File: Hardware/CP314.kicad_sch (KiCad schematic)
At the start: 14 parts, among them IC1 IS63WV1288DBLL-10TLI, IC2 SN74LVC573APWRE4, IC3 SN74LVC573APWRE4, J1 Raspberry_Pi_2_3, J2 Conn_02x11_Odd_Even, U1 XC9572XL-VQ64

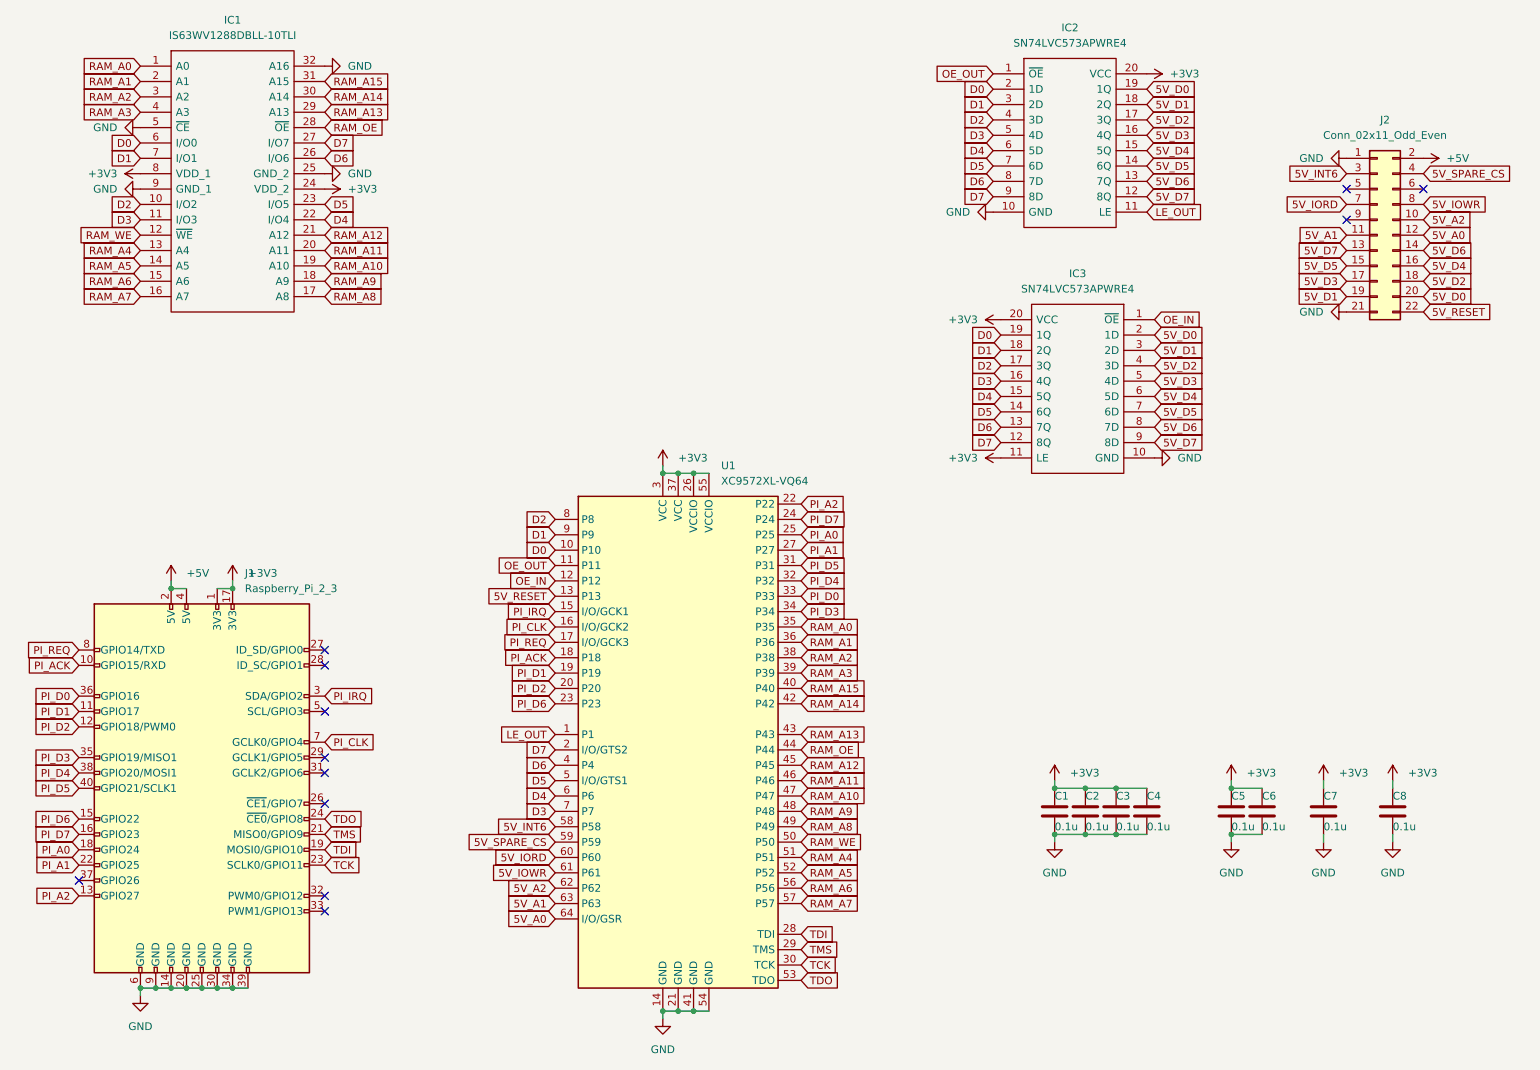
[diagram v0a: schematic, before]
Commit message: Initial file updates
PCB data replaced. Readme updated/simplified with further links to Niklas repo.
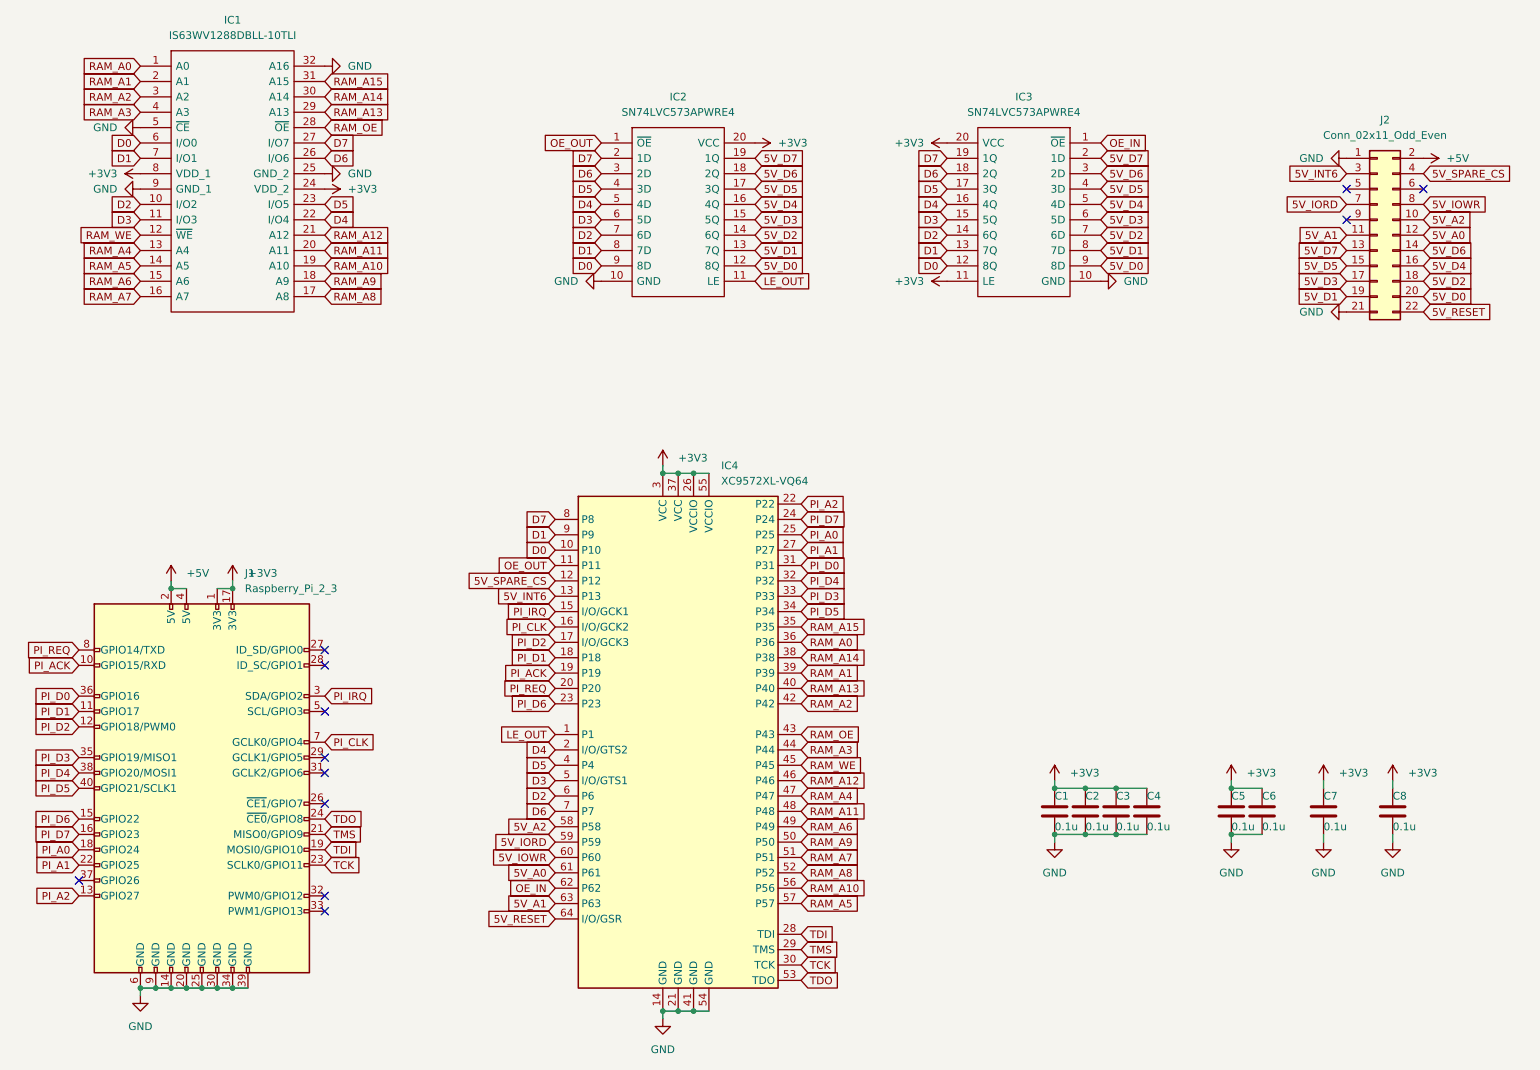
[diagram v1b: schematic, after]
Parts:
- IC1: footprint SOIC127P1176X120-32N -> Package_SO:TSOP-II-32_21.0x10.2mm_P1.27mm
- IC2, IC3: footprint SOP65P640X120-20N -> Package_SO:TSSOP-20_4.4x6.5mm_P0.65mm
- J1: footprint Connector_PinSocket_2.54mm:PinSocket_2x20_P2.54mm_Vertical -> Adafruit:ADA3708_RPI-ZERO_NO_HOLES; symbol Connector:Raspberry_Pi_2_3 -> Adafruit:Raspberry Pi; MANUFACTURER (none) -> Raspberry Pi Foundation
- J2: footprint Connector_PinSocket_2.00mm:PinSocket_2x11_P2.00mm_Vertical -> Connector_PinSocket_2.00mm:PinSocket_2x11_P2.00mm_Vertical_SMD
- renumbered U1 to IC4
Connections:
- net 5V_A0: now also IC4.61 (P61); no longer IC4.64 (I/O/GSR)
- net 5V_A2: now also IC4.58 (P58); no longer IC4.62 (P62)
- net 5V_D0: now also IC2.12 (8Q), IC3.9 (8D); no longer IC2.19 (1Q), IC3.2 (1D)
- net 5V_D1: now also IC2.13 (7Q), IC3.8 (7D); no longer IC2.18 (2Q), IC3.3 (2D)
- net 5V_D2: now also IC2.14 (6Q), IC3.7 (6D); no longer IC2.17 (3Q), IC3.4 (3D)
- net 5V_D3: now also IC2.15 (5Q), IC3.6 (5D); no longer IC2.16 (4Q), IC3.5 (4D)
- net 5V_D4: now also IC2.16 (4Q), IC3.5 (4D); no longer IC2.15 (5Q), IC3.6 (5D)
- net 5V_D5: now also IC2.17 (3Q), IC3.4 (3D); no longer IC2.14 (6Q), IC3.7 (6D)
- net 5V_D6: now also IC2.18 (2Q), IC3.3 (2D); no longer IC2.13 (7Q), IC3.8 (7D)
- net 5V_D7: now also IC2.19 (1Q), IC3.2 (1D); no longer IC2.12 (8Q), IC3.9 (8D)
- net 5V_INT6: now also IC4.13 (P13); no longer IC4.58 (P58)
- net 5V_IORD: now also IC4.59 (P59); no longer IC4.60 (P60)
- net 5V_IOWR: now also IC4.60 (P60); no longer IC4.61 (P61)
- net 5V_RESET: now also IC4.64 (I/O/GSR); no longer IC4.13 (P13)
- net 5V_SPARE_CS: now also IC4.12 (P12); no longer IC4.59 (P59)
- net D0: now also IC2.9 (8D), IC3.12 (8Q); no longer IC2.2 (1D), IC3.19 (1Q)
- net D1: now also IC2.8 (7D), IC3.13 (7Q); no longer IC2.3 (2D), IC3.18 (2Q)
- net D2: now also IC2.7 (6D), IC3.14 (6Q), IC4.6 (P6); no longer IC2.4 (3D), IC3.17 (3Q), IC4.8 (P8)
- net D3: now also IC2.6 (5D), IC3.15 (5Q), IC4.5 (I/O/GTS1); no longer IC2.5 (4D), IC3.16 (4Q), IC4.7 (P7)
- net D4: now also IC2.5 (4D), IC3.16 (4Q), IC4.2 (I/O/GTS2); no longer IC2.6 (5D), IC3.15 (5Q), IC4.6 (P6)
- net D5: now also IC2.4 (3D), IC3.17 (3Q), IC4.4 (P4); no longer IC2.7 (6D), IC3.14 (6Q), IC4.5 (I/O/GTS1)
- net D6: now also IC2.3 (2D), IC3.18 (2Q), IC4.7 (P7); no longer IC2.8 (7D), IC3.13 (7Q), IC4.4 (P4)
- net D7: now also IC2.2 (1D), IC3.19 (1Q), IC4.8 (P8); no longer IC2.9 (8D), IC3.12 (8Q), IC4.2 (I/O/GTS2)
- net OE_IN: now also IC4.62 (P62); no longer IC4.12 (P12)
- net PI_ACK: now also IC4.19 (P19); no longer IC4.18 (P18)
- net PI_D0: now also IC4.31 (P31); no longer IC4.33 (P33)
- net PI_D1: now also IC4.18 (P18); no longer IC4.19 (P19)
- net PI_D2: now also IC4.17 (I/O/GCK3); no longer IC4.20 (P20)
- net PI_D3: now also IC4.33 (P33); no longer IC4.34 (P34)
- net PI_D5: now also IC4.34 (P34); no longer IC4.31 (P31)
- net PI_REQ: now also IC4.20 (P20); no longer IC4.17 (I/O/GCK3)
- net RAM_A0: now also IC4.36 (P36); no longer IC4.35 (P35)
- net RAM_A1: now also IC4.39 (P39); no longer IC4.36 (P36)
- net RAM_A10: now also IC4.56 (P56); no longer IC4.47 (P47)
- net RAM_A11: now also IC4.48 (P48); no longer IC4.46 (P46)
- net RAM_A12: now also IC4.46 (P46); no longer IC4.45 (P45)
- net RAM_A13: now also IC4.40 (P40); no longer IC4.43 (P43)
- net RAM_A14: now also IC4.38 (P38); no longer IC4.42 (P42)
- net RAM_A15: now also IC4.35 (P35); no longer IC4.40 (P40)
- net RAM_A2: now also IC4.42 (P42); no longer IC4.38 (P38)
- net RAM_A3: now also IC4.44 (P44); no longer IC4.39 (P39)
- net RAM_A4: now also IC4.47 (P47); no longer IC4.51 (P51)
- net RAM_A5: now also IC4.57 (P57); no longer IC4.52 (P52)
- net RAM_A6: now also IC4.49 (P49); no longer IC4.56 (P56)
- net RAM_A7: now also IC4.51 (P51); no longer IC4.57 (P57)
- net RAM_A8: now also IC4.52 (P52); no longer IC4.49 (P49)
- net RAM_A9: now also IC4.50 (P50); no longer IC4.48 (P48)
- net RAM_OE: now also IC4.43 (P43); no longer IC4.44 (P44)
- net RAM_WE: now also IC4.45 (P45); no longer IC4.50 (P50)
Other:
- moved on the sheet: IC2, IC3
